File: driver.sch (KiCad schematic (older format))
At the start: 57 parts, among them U10 LM5008MM, U11 SN74LVC1G66DBVR, U12 2ED2304S06F, U13 SN74LVC1G66DBVR, U14 AQY282S, U15 2ED2304S06F, U17 LMR12010YMKE, U2 SN74LVC1G66DBVR, U3 2ED2304S06F

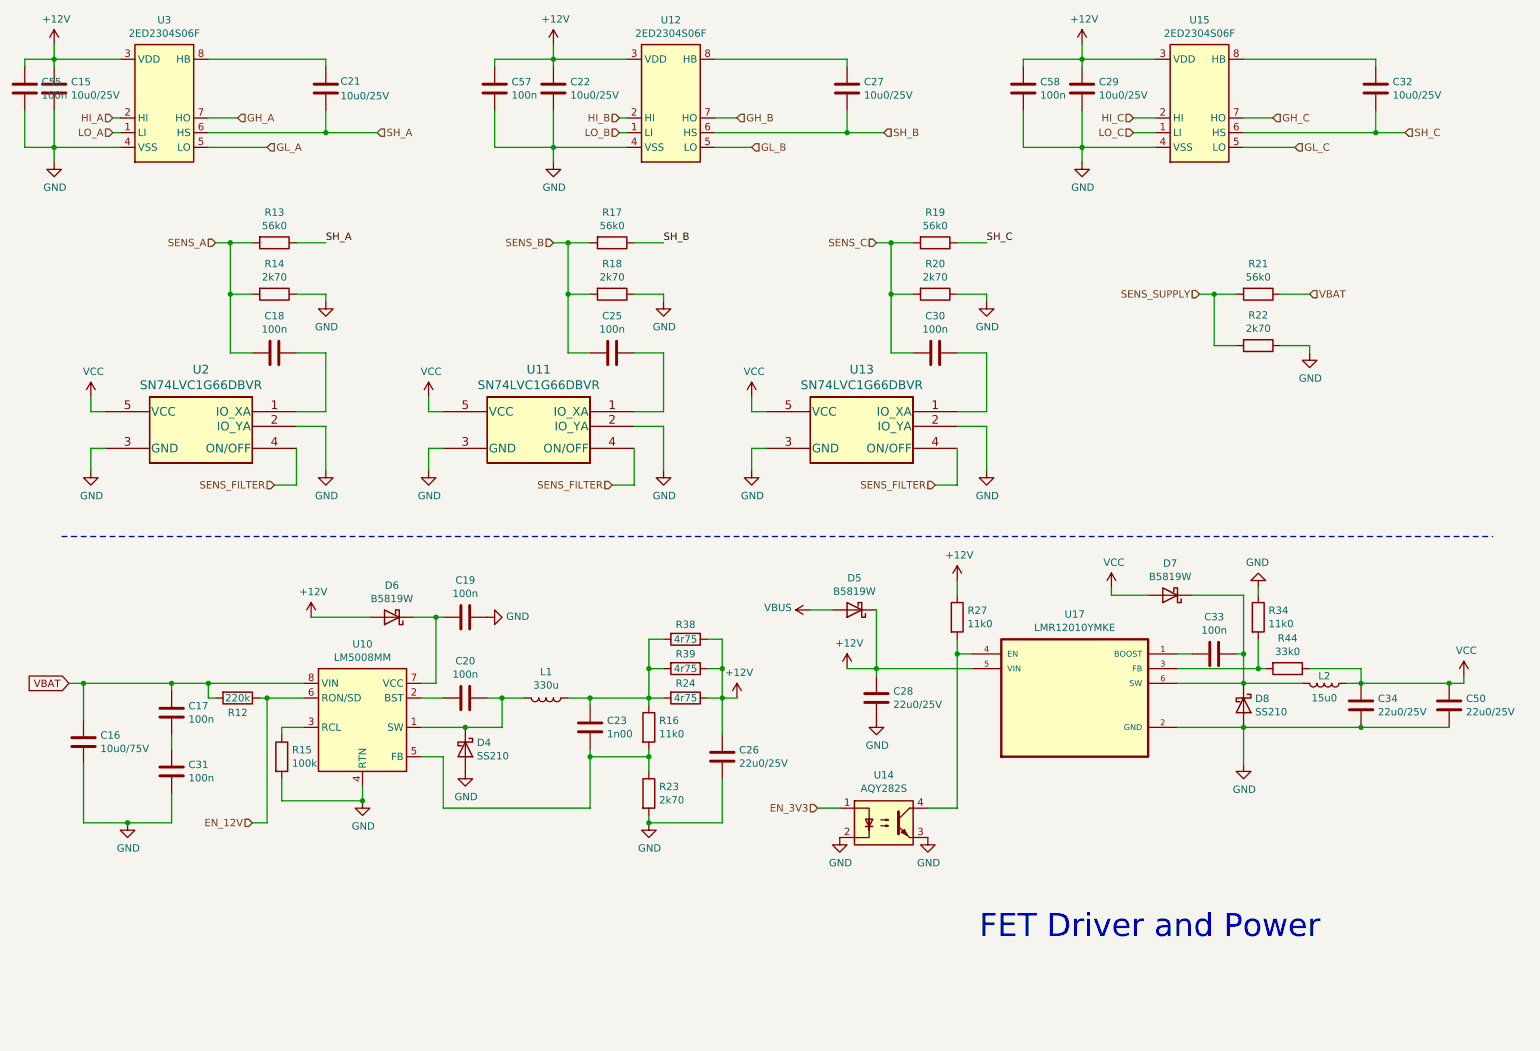
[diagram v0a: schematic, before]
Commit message: save
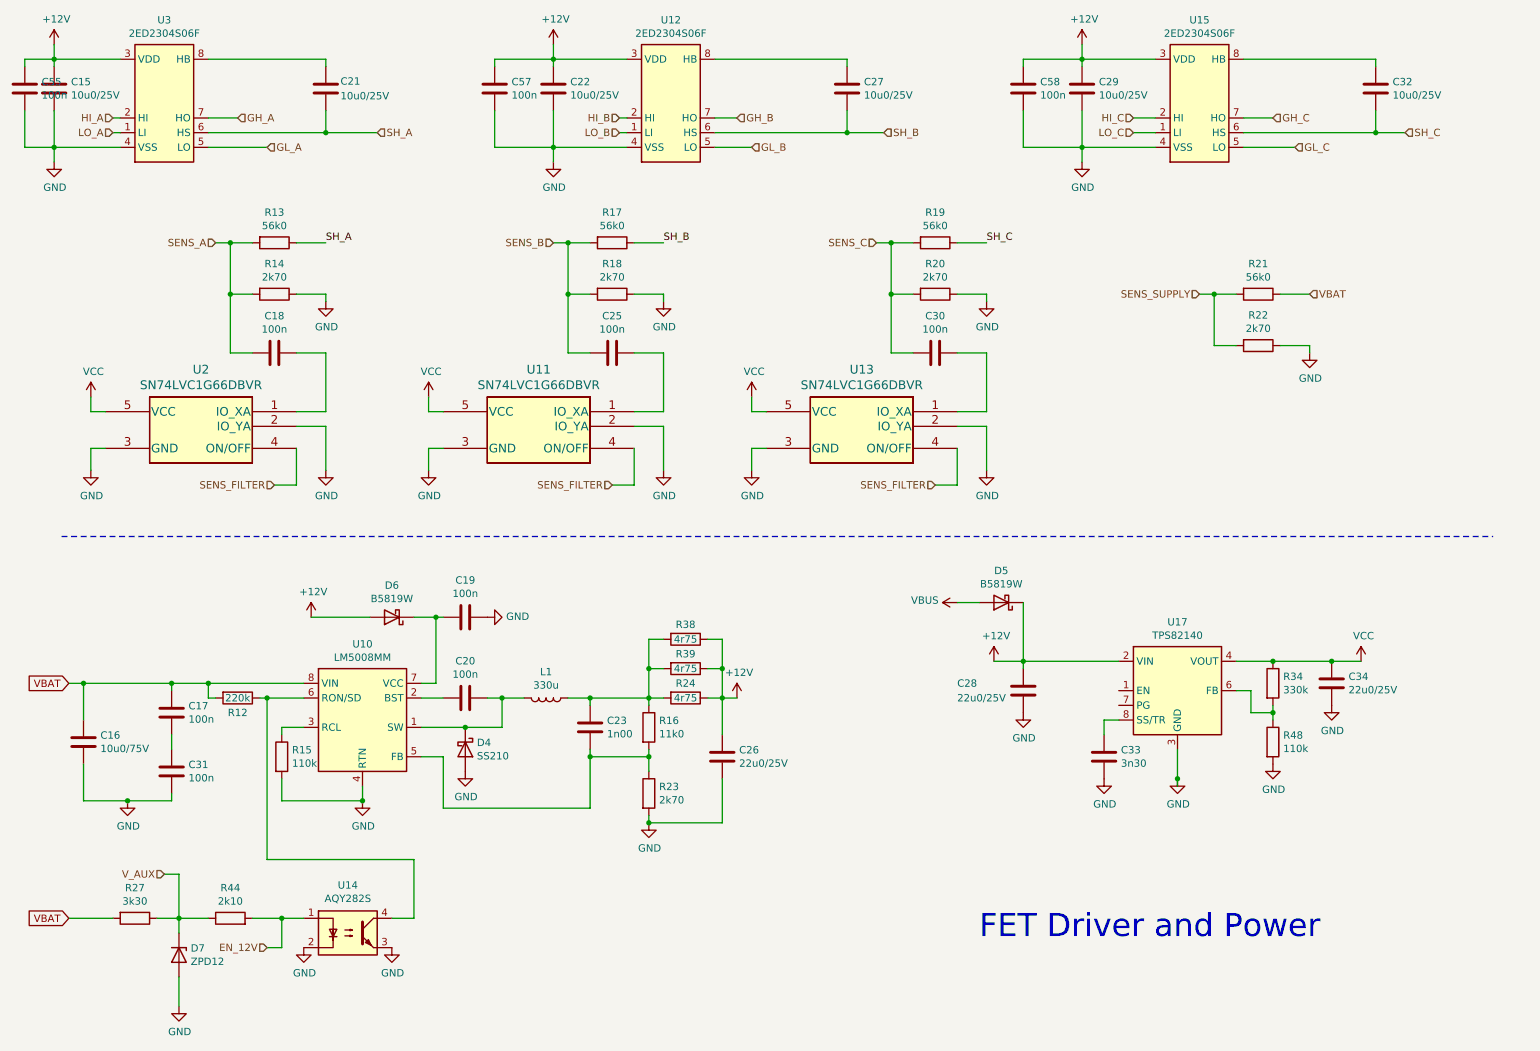
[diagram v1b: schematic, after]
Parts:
- removed C50: 22u0/25V, Capacitor_SMD:C_0805_2012Metric, symbol Device:C
- removed D7: B5819W, Diode_SMD:D_SOD-123, symbol Device:D_Schottky
- removed D8: SS210, Diode_SMD:D_SMA, symbol Diode:B360
- removed L2: 15u0, Inductor_SMD:L_6.3x6.3_H3, symbol Device:L
- removed U17: LMR12010YMKE, gesc:SOT95P280X110-6N, symbol gesc:LMR12010YMKE_NOPB
- added D7: ZPD12, Diode_SMD:D_MiniMELF, symbol Diode:ZPDxx
- added R48: 110k, Resistor_SMD:R_0805_2012Metric, symbol Device:R
- added U17: TPS82140, Package_LGA:Texas_SIL0008D_MicroSiP-8-1EP_2.8x3mm_P0.65mm_EP1.1x1.9mm, symbol Regulator_Switching:TPS82140
- C33: value 100n -> 3n30
- R15: value 100k -> 110k
- R27: value 11k0 -> 3k30
- R34: value 11k0 -> 330k
- R44: value 33k0 -> 2k10
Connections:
- net EN_3V3 is gone; now on net EN_12V: U14.1
- net +12V: now also U17.2 (VIN); no longer R27.1
- net EN_12V: now also R44.2; no longer R12.1, U10.6 (RON/SD)
- net GND: now also C33.2, D7.2 (A), R48.2, U17.3 (GND), U17.9 (GND); no longer R34.1
- net VBAT: now also R27.2
- net VCC: now also R34.1, U17.4 (VOUT), U17.5 (VOUT); no longer R44.1
- net at U14.4: now also R12.1, U10.6 (RON/SD); no longer R27.2
- net at C33.1: now also U17.8 (SS/TR)
- net at R34.2: now also R48.1, U17.6 (FB); no longer R44.2
- new net V_AUX: D7.1 (K), R27.1, R44.1
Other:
- moved on the sheet: C28, C34, D5, R34, U14

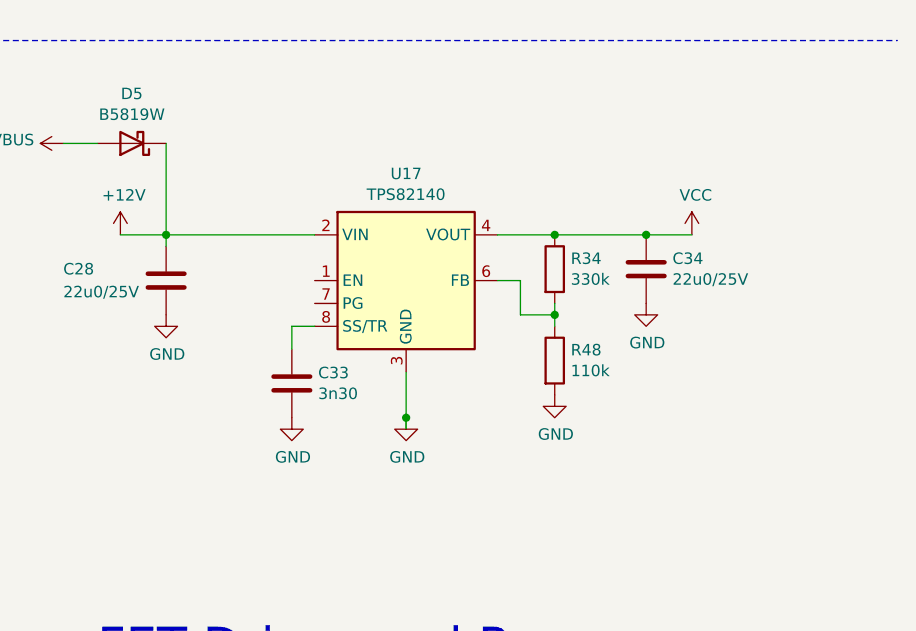
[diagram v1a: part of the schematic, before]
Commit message: Version rund platziert
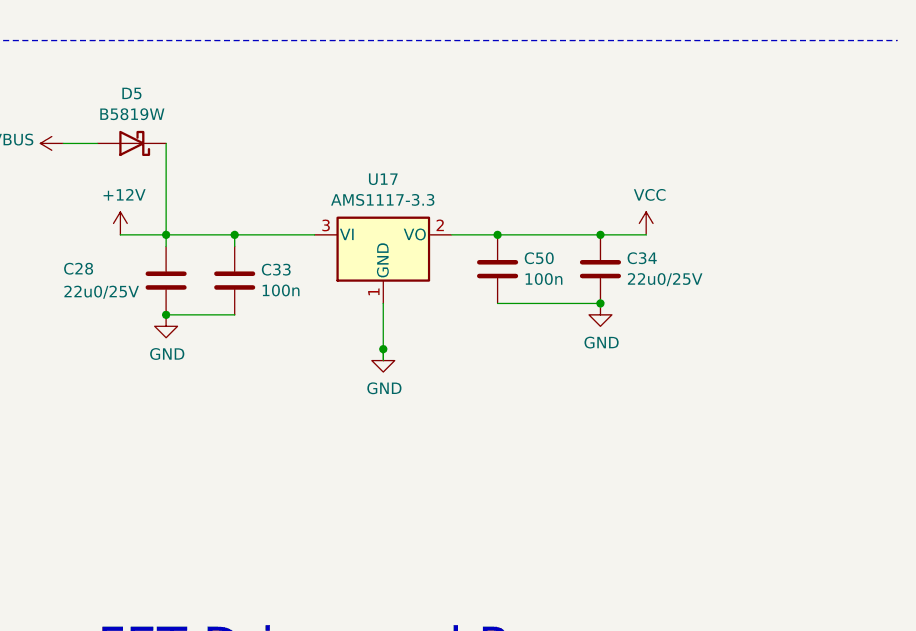
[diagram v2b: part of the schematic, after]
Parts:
- removed R34: 330k, Resistor_SMD:R_0805_2012Metric, symbol Device:R
- removed R48: 110k, Resistor_SMD:R_0805_2012Metric, symbol Device:R
- removed U17: TPS82140, Package_LGA:Texas_SIL0008D_MicroSiP-8-1EP_2.8x3mm_P0.65mm_EP1.1x1.9mm, symbol Regulator_Switching:TPS82140
- added C50: 100n, Capacitor_SMD:C_0805_2012Metric, symbol Device:C
- added U17: AMS1117-3.3, Package_TO_SOT_SMD:SOT-223-3_TabPin2, symbol Regulator_Linear:AMS1117-3.3
- C33: value 3n30 -> 100n
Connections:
- net +12V: now also C33.1, U17.3 (VI)
- net GND: now also C50.2, U17.1 (GND)
- net VCC: now also C50.1, U17.2 (VO)
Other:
- moved on the sheet: C34
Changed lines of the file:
@@
 L power:VCC #PWR0152
 U 1 1 5EB2A2D9
-P 9750 5050
-F 0 "#PWR0152" H 9750 4900 50  0001 C CNN
-F 1 "VCC" H 9767 5223 50  0000 C CNN
-F 2 "" H 9750 5050 50  0001 C CNN
-F 3 "" H 9750 5050 50  0001 C CNN
-	1    9750 5050
+P 9550 5050
+F 0 "#PWR0152" H 9550 4900 50  0001 C CNN
+F 1 "VCC" H 9567 5223 50  0000 C CNN
+F 2 "" H 9550 5050 50  0001 C CNN
+F 3 "" H 9550 5050 50  0001 C CNN
+	1    9550 5050
 	1    0    0    -1
 $EndComp
@@
 L Device:C C34
 U 1 1 601ECA0B
-P 9550 5200
-F 0 "C34" H 9665 5246 50  0000 L CNN
-F 1 "22u0/25V" H 9665 5155 50  0000 L CNN
-F 2 "Capacitor_SMD:C_0805_2012Metric" H 9588 5050 50  0001 C CNN
-F 3 "~" H 9550 5200 50  0001 C CNN
-	1    9550 5200
-	1    0    0    -1
-$EndComp
-$Comp
-L Device:R R34
-U 1 1 6026DD04
-P 9150 5200
-F 0 "R34" H 9220 5246 50  0000 L CNN
-F 1 "330k" H 9220 5155 50  0000 L CNN
-F 2 "Resistor_SMD:R_0805_2012Metric" V 9080 5200 50  0001 C CNN
-F 3 "~" H 9150 5200 50  0001 C CNN
-	1    9150 5200
+P 9350 5200
+F 0 "C34" H 9465 5246 50  0000 L CNN
+F 1 "22u0/25V" H 9465 5155 50  0000 L CNN
+F 2 "Capacitor_SMD:C_0805_2012Metric" H 9388 5050 50  0001 C CNN
+F 3 "~" H 9350 5200 50  0001 C CNN
+	1    9350 5200
 	1    0    0    -1
 $EndComp
@@
 Wire Wire Line
 	7450 1550 7850 1550
-$Comp
-L Regulator_Switching:TPS82140 U17
-U 1 1 6042CA52
-P 8500 5250
-F 0 "U17" H 8500 5717 50  0000 C CNN
-F 1 "TPS82140" H 8500 5626 50  0000 C CNN
-F 2 "Package_LGA:Texas_SIL0008D_MicroSiP-8-1EP_2.8x3mm_P0.65mm_EP1.1x1.9mm" H 8500 4600 50  0001 C CNN
-F 3 "http://www.ti.com/lit/ds/symlink/tps82140.pdf" H 8500 4500 50  0001 C CNN
-	1    8500 5250
-	1    0    0    -1
-$EndComp
-$Comp
-L Device:C C33
-U 1 1 6046F0F7
-P 8000 5700
-F 0 "C33" H 8115 5746 50  0000 L CNN
-F 1 "3n30" H 8115 5655 50  0000 L CNN
-F 2 "Capacitor_SMD:C_0805_2012Metric" H 8038 5550 50  0001 C CNN
-F 3 "~" H 8000 5700 50  0001 C CNN
-	1    8000 5700
-	1    0    0    -1
-$EndComp
-Wire Wire Line
-	8000 5550 8000 5450
-Wire Wire Line
-	8000 5450 8100 5450
-Wire Wire Line
-	8500 5650 8500 5850
+Wire Wire Line
+	8400 5350 8400 5550
 $Comp
 L power:GND #PWR0151
 U 1 1 604A639D
-P 8500 5850
-F 0 "#PWR0151" H 8500 5600 50  0001 C CNN
-F 1 "GND" H 8505 5677 50  0000 C CNN
-F 2 "" H 8500 5850 50  0001 C CNN
-F 3 "" H 8500 5850 50  0001 C CNN
-	1    8500 5850
-	1    0    0    -1
-$EndComp
-$Comp
-L power:GND #PWR0160
-U 1 1 604A67D5
-P 8000 5850
-F 0 "#PWR0160" H 8000 5600 50  0001 C CNN
-F 1 "GND" H 8005 5677 50  0000 C CNN
-F 2 "" H 8000 5850 50  0001 C CNN
-F 3 "" H 8000 5850 50  0001 C CNN
-	1    8000 5850
-	1    0    0    -1
-$EndComp
-Connection ~ 8500 5850
-Wire Wire Line
-	8500 5850 8500 5900
-$Comp
-L Device:R R48
-U 1 1 604AC2B0
-P 9150 5600
-F 0 "R48" H 9220 5646 50  0000 L CNN
-F 1 "110k" H 9220 5555 50  0000 L CNN
-F 2 "Resistor_SMD:R_0805_2012Metric" V 9080 5600 50  0001 C CNN
-F 3 "~" H 9150 5600 50  0001 C CNN
-	1    9150 5600
-	1    0    0    -1
-$EndComp
-Wire Wire Line
-	9150 5350 9150 5400
-Wire Wire Line
-	8900 5250 9000 5250
-Wire Wire Line
-	9000 5250 9000 5400
-Wire Wire Line
-	9000 5400 9150 5400
-Connection ~ 9150 5400
-Wire Wire Line
-	9150 5400 9150 5450
-$Comp
-L power:GND #PWR0161
-U 1 1 604C80AE
-P 9150 5750
-F 0 "#PWR0161" H 9150 5500 50  0001 C CNN
-F 1 "GND" H 9155 5577 50  0000 C CNN
-F 2 "" H 9150 5750 50  0001 C CNN
-F 3 "" H 9150 5750 50  0001 C CNN
-	1    9150 5750
-	1    0    0    -1
-$EndComp
-Wire Wire Line
-	8900 5050 9150 5050
-Wire Wire Line
-	9150 5050 9550 5050
-Connection ~ 9150 5050
-Wire Wire Line
-	9550 5050 9750 5050
-Connection ~ 9550 5050
+P 8400 5550
+F 0 "#PWR0151" H 8400 5300 50  0001 C CNN
+F 1 "GND" H 8405 5377 50  0000 C CNN
+F 2 "" H 8400 5550 50  0001 C CNN
+F 3 "" H 8400 5550 50  0001 C CNN
+	1    8400 5550
+	1    0    0    -1
+$EndComp
+Connection ~ 8400 5550
+Wire Wire Line
+	8400 5550 8400 5600
+Wire Wire Line
+	9350 5050 9550 5050
+Connection ~ 9350 5050
 Wire Wire Line
 	3300 6800 3150 6800
 Wire Wire Line
-	7450 5050 8100 5050
+	7450 5050 7750 5050
 Wire Wire Line
 	2300 5300 2300 6400
@@
 L power:GND #PWR0168
 U 1 1 607144C0
-P 9550 5350
-F 0 "#PWR0168" H 9550 5100 50  0001 C CNN
-F 1 "GND" H 9555 5177 50  0000 C CNN
-F 2 "" H 9550 5350 50  0001 C CNN
-F 3 "" H 9550 5350 50  0001 C CNN
-	1    9550 5350
-	1    0    0    -1
-$EndComp
+P 9350 5350
+F 0 "#PWR0168" H 9350 5100 50  0001 C CNN
+F 1 "GND" H 9355 5177 50  0000 C CNN
+F 2 "" H 9350 5350 50  0001 C CNN
+F 3 "" H 9350 5350 50  0001 C CNN
+	1    9350 5350
+	1    0    0    -1
+$EndComp
+$Comp
+L Regulator_Linear:AMS1117-3.3 U17
+U 1 1 60438DE9
+P 8400 5050
+F 0 "U17" H 8400 5292 50  0000 C CNN
+F 1 "AMS1117-3.3" H 8400 5201 50  0000 C CNN
+F 2 "Package_TO_SOT_SMD:SOT-223-3_TabPin2" H 8400 5250 50  0001 C CNN
+F 3 "http://www.advanced-monolithic.com/pdf/ds1117.pdf" H 8500 4800 50  0001 C CNN
+	1    8400 5050
+	1    0    0    -1
+$EndComp
+Wire Wire Line
+	8700 5050 8900 5050
+$Comp
+L Device:C C33
+U 1 1 6048B400
+P 7750 5250
+F 0 "C33" H 7865 5296 50  0000 L CNN
+F 1 "100n" H 7865 5205 50  0000 L CNN
+F 2 "Capacitor_SMD:C_0805_2012Metric" H 7788 5100 50  0001 C CNN
+F 3 "~" H 7750 5250 50  0001 C CNN
+	1    7750 5250
+	1    0    0    -1
+$EndComp
+Wire Wire Line
+	7750 5100 7750 5050
+Connection ~ 7750 5050
+Wire Wire Line
+	7750 5050 8100 5050
+Wire Wire Line
+	7750 5400 7450 5400
+Connection ~ 7450 5400
+$Comp
+L Device:C C50
+U 1 1 604A6BBB
+P 8900 5200
+F 0 "C50" H 9015 5246 50  0000 L CNN
+F 1 "100n" H 9015 5155 50  0000 L CNN
+F 2 "Capacitor_SMD:C_0805_2012Metric" H 8938 5050 50  0001 C CNN
+F 3 "~" H 8900 5200 50  0001 C CNN
+	1    8900 5200
+	1    0    0    -1
+$EndComp
+Connection ~ 8900 5050
+Wire Wire Line
+	8900 5050 9350 5050
+Wire Wire Line
+	8900 5350 9350 5350
+Connection ~ 9350 5350
 $EndSCHEMATC
